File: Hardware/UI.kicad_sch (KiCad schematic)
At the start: 53 parts, among them J101 USB_C_Receptacle_USB2.0_16P, J102 ST7789 LCD, J103 TC2030, J104 Expansion, Q101 AO3400A, SW101 SIQ-02FVS3, SW102 SW_Back, SW103 Reset, SW104 Boot, U101 CH32X035G8U6, U102 AP2112K-3.3, U103 TPS22915CYFPR, U104 SIT3088ETK, U105 LIS3DH

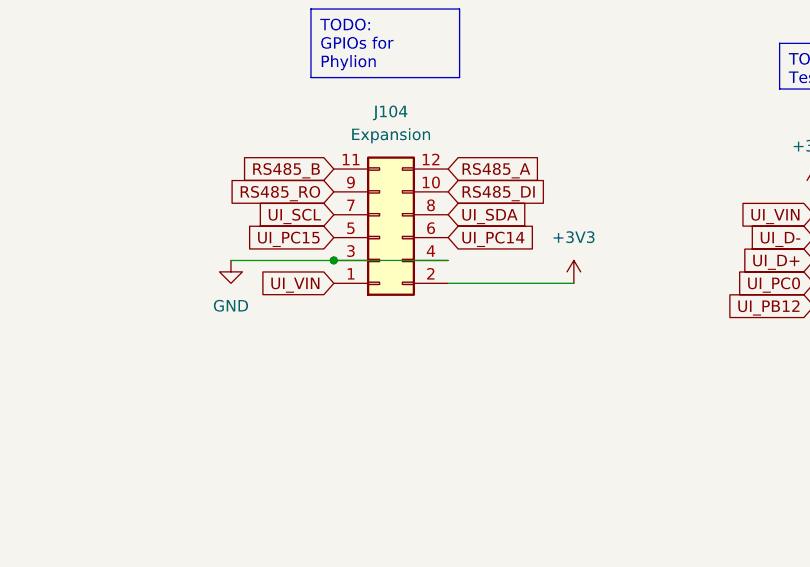
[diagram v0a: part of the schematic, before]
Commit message: final tweaks before routing traces
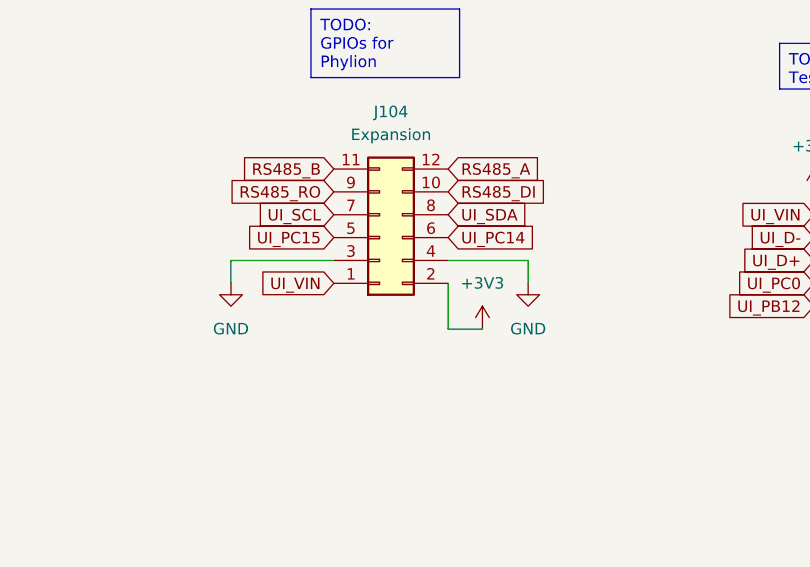
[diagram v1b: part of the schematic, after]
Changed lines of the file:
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@@
 	)
 	(junction
-		(at 199.39 157.48)
-		(diameter 0)
-		(color 0 0 0 0)
-	)
-	(junction
 		(at 219.71 97.79)
 		(diameter 0)
@@
 	(wire
 		(pts
-			(xy 199.39 157.48) (xy 212.09 157.48)
+			(xy 109.22 128.27) (xy 109.22 127)
 		)
 		(stroke
@@
 	(wire
 		(pts
-			(xy 109.22 128.27) (xy 109.22 127)
+			(xy 271.78 153.67) (xy 271.78 158.75)
 		)
 		(stroke
@@
 	(wire
 		(pts
-			(xy 271.78 153.67) (xy 271.78 158.75)
+			(xy 256.54 106.68) (xy 265.43 106.68)
 		)
 		(stroke
@@
 	(wire
 		(pts
-			(xy 256.54 106.68) (xy 265.43 106.68)
+			(xy 187.96 160.02) (xy 187.96 157.48)
 		)
 		(stroke
@@
 	(wire
 		(pts
+			(xy 187.96 157.48) (xy 199.39 157.48)
+		)
+		(stroke
+			(width 0)
+			(type default)
+		)
+	)
+	(wire
+		(pts
 			(xy 16.51 115.57) (xy 20.32 115.57)
 		)
@@
 	(wire
 		(pts
+			(xy 220.98 160.02) (xy 220.98 157.48)
+		)
+		(stroke
+			(width 0)
+			(type default)
+		)
+	)
+	(wire
+		(pts
 			(xy 116.84 180.34) (xy 119.38 180.34)
 		)
@@
 	(wire
 		(pts
+			(xy 212.09 157.48) (xy 220.98 157.48)
+		)
+		(stroke
+			(width 0)
+			(type default)
+		)
+	)
+	(wire
+		(pts
 			(xy 256.54 73.66) (xy 256.54 74.93)
 		)
@@
 	(wire
 		(pts
+			(xy 212.09 165.1) (xy 212.09 160.02)
+		)
+		(stroke
+			(width 0)
+			(type default)
+		)
+	)
+	(wire
+		(pts
 			(xy 247.65 26.67) (xy 256.54 26.67)
 		)
@@
 	(wire
 		(pts
-			(xy 212.09 160.02) (xy 226.06 160.02)
+			(xy 212.09 165.1) (xy 215.9 165.1)
 		)
 		(stroke
@@
 	(wire
 		(pts
-			(xy 187.96 157.48) (xy 199.39 157.48)
-		)
-		(stroke
-			(width 0)
-			(type default)
-		)
-	)
-	(wire
-		(pts
 			(xy 234.95 72.39) (xy 234.95 81.28)
 		)
@@
 	(label "UI_D-"
 		(at 66.04 41.91 0)
-		(fields_autoplaced yes)
 		(effects
 			(font
@@
 	(label "UI_VIN"
 		(at 29.21 124.46 0)
-		(fields_autoplaced yes)
 		(effects
 			(font
@@
 	(label "UI_D+"
 		(at 66.04 44.45 0)
-		(fields_autoplaced yes)
 		(effects
 			(font
@@
 		(shape input)
 		(at 151.13 67.31 0)
-		(fields_autoplaced yes)
 		(effects
 			(font
@@
 		(shape input)
 		(at 151.13 69.85 0)
-		(fields_autoplaced yes)
 		(effects
 			(font
@@
 	(symbol
 		(lib_id "power:+3V3")
-		(at 226.06 160.02 0)
+		(at 215.9 165.1 0)
 		(unit 1)
 		(exclude_from_sim no)
@@
 		(fields_autoplaced yes)
 		(property "Reference" "#PWR0135"
-			(at 226.06 163.83 0)
+			(at 215.9 168.91 0)
 			(effects
 				(font
@@
 		)
 		(property "Value" "+3V3"
-			(at 226.06 154.94 0)
+			(at 215.9 160.02 0)
 			(effects
 				(font
@@
 		)
 		(property "Footprint" ""
-			(at 226.06 160.02 0)
+			(at 215.9 165.1 0)
 			(effects
 				(font
@@
 		)
 		(property "Datasheet" ""
-			(at 226.06 160.02 0)
+			(at 215.9 165.1 0)
 			(effects
 				(font
@@
 		)
 		(property "Description" "Power symbol creates a global label with name \"+3V3\""
-			(at 226.06 160.02 0)
+			(at 215.9 165.1 0)
 			(effects
 				(font
@@
 	(symbol
 		(lib_id "power:GND")
-		(at 187.96 157.48 0)
+		(at 187.96 160.02 0)
 		(unit 1)
 		(exclude_from_sim no)
@@
 		(fields_autoplaced yes)
 		(property "Reference" "#PWR0136"
-			(at 187.96 163.83 0)
+			(at 187.96 166.37 0)
 			(effects
 				(font
@@
 		)
 		(property "Value" "GND"
-			(at 187.96 162.56 0)
+			(at 187.96 165.1 0)
 			(effects
 				(font
@@
 		)
 		(property "Footprint" ""
-			(at 187.96 157.48 0)
+			(at 187.96 160.02 0)
 			(effects
 				(font
@@
 		)
 		(property "Datasheet" ""
-			(at 187.96 157.48 0)
+			(at 187.96 160.02 0)
 			(effects
 				(font
@@
 		)
 		(property "Description" "Power symbol creates a global label with name \"GND\" , ground"
-			(at 187.96 157.48 0)
+			(at 187.96 160.02 0)
 			(effects
 				(font
@@
 					(unit 1)
 				)
+			)
+		)
+	)
+	(symbol
+		(lib_id "power:GND")
+		(at 220.98 160.02 0)
+		(unit 1)
+		(exclude_from_sim no)
+		(in_bom yes)
+		(on_board yes)
+		(dnp no)
+		(fields_autoplaced yes)
+		(property "Reference" "#PWR0149"
+			(at 220.98 166.37 0)
+			(effects
+				(font
+					(size 1.27 1.27)
+				)
+				(hide yes)
+			)
+		)
+		(property "Value" "GND"
+			(at 220.98 165.1 0)
+			(effects
+				(font
+					(size 1.27 1.27)
+				)
+			)
+		)
+		(property "Footprint" ""
+			(at 220.98 160.02 0)
+			(effects
+				(font
+					(size 1.27 1.27)
+				)
+				(hide yes)
+			)
+		)
+		(property "Datasheet" ""
+			(at 220.98 160.02 0)
+			(effects
+				(font
+					(size 1.27 1.27)
+				)
+				(hide yes)
+			)
+		)
+		(property "Description" "Power symbol creates a global label with name \"GND\" , ground"
+			(at 220.98 160.02 0)
+			(effects
+				(font
+					(size 1.27 1.27)
+				)
+				(hide yes)
+			)
+		)
+		(pin "1"
+		)
+		(instances
+			(project "USB-C PSU"
+				(path "/2795a064-4b14-4857-8c9a-fd2d32a5a222/83a45ffb-89fc-4bf0-b371-2eda7791aa05"
+					(reference "#PWR0149")
+					(unit 1)
+				)
